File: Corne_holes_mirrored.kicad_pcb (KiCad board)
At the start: 2 copper layers, 133.7 x 91.4 mm, 48 parts, among them J1 MJ-4PP-9, J2 OLED, SW1 SW_PUSH, SW10 SW_PUSH, SW11 SW_PUSH, SW12 SW_PUSH, SW13 SW_PUSH, SW14 SW_PUSH, SW15 SW_PUSH, SW16 SW_PUSH, SW17 SW_PUSH, SW18 SW_PUSH, SW19 SW_PUSH, SW2 SW_PUSH, SW20 SW_PUSH, SW3 SW_PUSH, SW4 SW_PUSH, SW5 SW_PUSH, SW6 SW_PUSH, SW7 SW_PUSH, SW8 SW_PUSH, SW9 SW_PUSH, U1 ProMicro

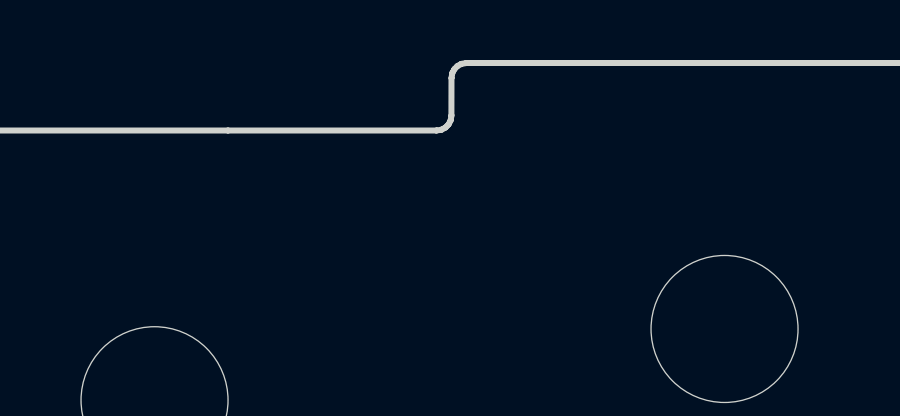
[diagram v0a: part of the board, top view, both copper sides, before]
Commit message: Fix issues, add step file
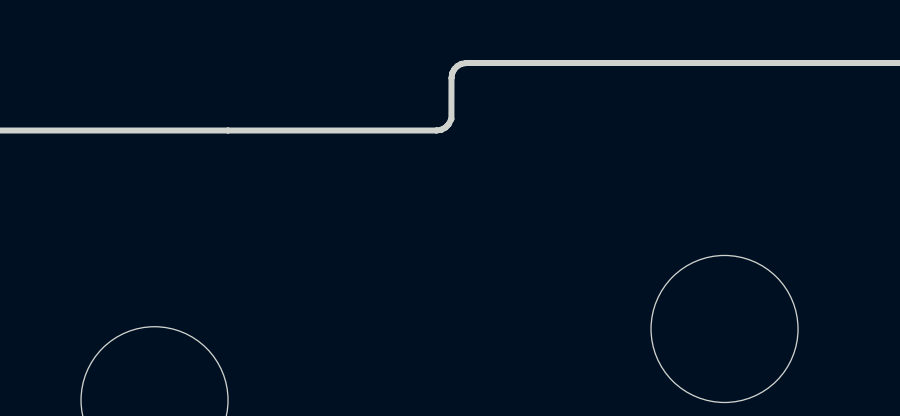
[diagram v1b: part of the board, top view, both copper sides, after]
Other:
- outline, holes or cut-outs redrawn
- net class Default removed
